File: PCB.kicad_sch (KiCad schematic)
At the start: 57 parts, among them J1 USB_C_Receptacle_USB2.0_16P, J10 Conn_01x05_Pin, J11 Conn_01x05_Pin, J12 Conn_01x03_Pin, J2 Conn_01x04_Pin, J3 Conn_01x04_Pin, J4 Conn_01x07_Pin, J5 Conn_01x02_Pin, J6 Conn_01x02_Pin, J7 Conn_01x02_Pin, J8 Conn_01x04_Pin, J9 Conn_01x07_Pin, SW1 SW_Push, SW2 SW_Push, U1 TMC2209_SILENTSTEPSTICK, U2 TMC2209_SILENTSTEPSTICK, U3 D3V3XA4B10LP, U4 AMS1117-3.3 (UMW), U5 TMC2209_SILENTSTEPSTICK, U6 ESP32-S3-WROOM-1

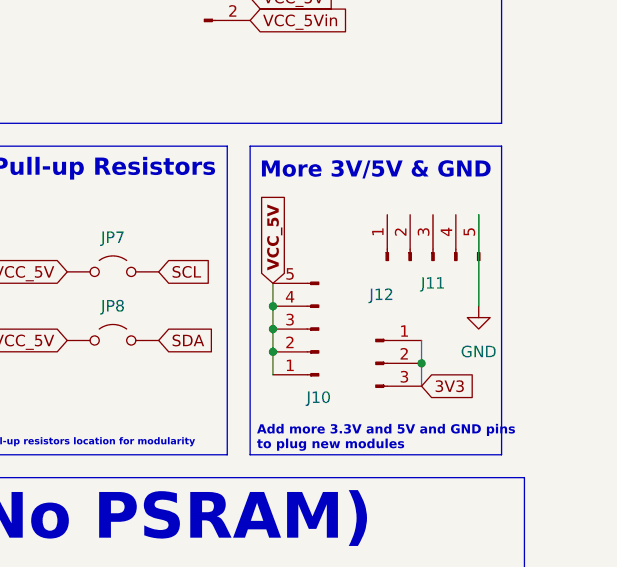
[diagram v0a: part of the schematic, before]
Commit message: Dernier DRC après modicifications
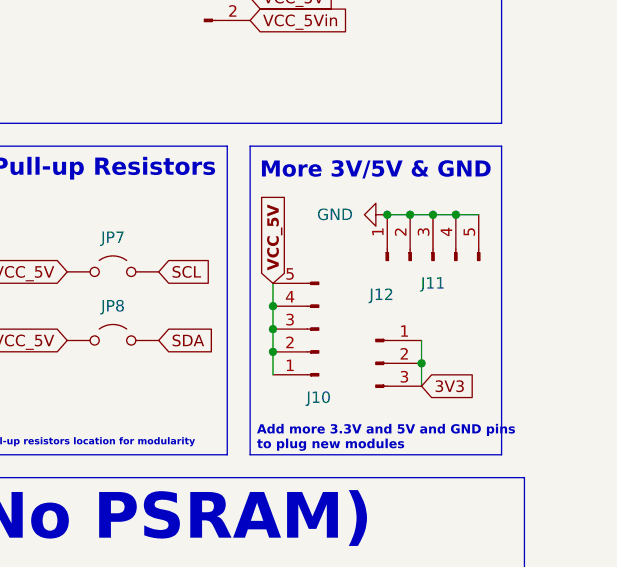
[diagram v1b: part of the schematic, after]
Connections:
- net GND: now also J11.1 (Pin_1), J11.2 (Pin_2), J11.3 (Pin_3), J11.4 (Pin_4)
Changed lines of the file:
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@@
 	)
 	(junction
+		(at 393.7 130.81)
+		(diameter 0)
+		(color 0 0 0 0)
+	)
+	(junction
 		(at 373.38 146.05)
 		(diameter 0)
@@
 	)
 	(junction
+		(at 386.08 130.81)
+		(diameter 0)
+		(color 0 0 0 0)
+	)
+	(junction
 		(at 290.83 176.53)
 		(diameter 0)
@@
 	)
 	(junction
+		(at 388.62 130.81)
+		(diameter 0)
+		(color 0 0 0 0)
+	)
+	(junction
 		(at 64.77 149.86)
 		(diameter 0)
@@
 	)
 	(junction
+		(at 391.16 130.81)
+		(diameter 0)
+		(color 0 0 0 0)
+	)
+	(junction
 		(at 373.38 143.51)
 		(diameter 0)
@@
 	(wire
 		(pts
+			(xy 388.62 130.81) (xy 391.16 130.81)
+		)
+		(stroke
+			(width 0)
+			(type default)
+		)
+	)
+	(wire
+		(pts
 			(xy 71.12 222.25) (xy 80.01 222.25)
 		)
@@
 	(wire
 		(pts
+			(xy 386.08 130.81) (xy 388.62 130.81)
+		)
+		(stroke
+			(width 0)
+			(type default)
+		)
+	)
+	(wire
+		(pts
 			(xy 71.12 222.25) (xy 71.12 223.52)
 		)
@@
 	(wire
 		(pts
+			(xy 393.7 130.81) (xy 396.24 130.81)
+		)
+		(stroke
+			(width 0)
+			(type default)
+		)
+	)
+	(wire
+		(pts
 			(xy 181.61 233.68) (xy 189.23 233.68)
 		)
@@
 	(wire
 		(pts
+			(xy 391.16 130.81) (xy 393.7 130.81)
+		)
+		(stroke
+			(width 0)
+			(type default)
+		)
+	)
+	(wire
+		(pts
 			(xy 74.93 58.42) (xy 80.01 58.42)
 		)
@@
 	(wire
 		(pts
-			(xy 396.24 130.81) (xy 396.24 140.97)
-		)
-		(stroke
-			(width 0)
-			(type default)
-		)
-	)
-	(wire
-		(pts
 			(xy 34.29 124.46) (xy 39.37 124.46)
 		)
@@
 	(symbol
 		(lib_id "power:GND")
-		(at 396.24 140.97 0)
+		(at 386.08 130.81 270)
 		(unit 1)
 		(exclude_from_sim no)
@@
 		(fields_autoplaced yes)
 		(property "Reference" "#PWR033"
-			(at 396.24 147.32 0)
+			(at 379.73 130.81 0)
 			(effects
 				(font
@@
 		)
 		(property "Value" "GND"
-			(at 396.24 146.05 0)
+			(at 382.27 130.8099 90)
 			(effects
 				(font
 					(size 1.27 1.27)
 				)
+				(justify right)
 			)
 		)
 		(property "Footprint" ""
-			(at 396.24 140.97 0)
+			(at 386.08 130.81 0)
 			(effects
 				(font
@@
 		)
 		(property "Datasheet" ""
-			(at 396.24 140.97 0)
+			(at 386.08 130.81 0)
 			(effects
 				(font
@@
 		)
 		(property "Description" "Power symbol creates a global label with name \"GND\" , ground"
-			(at 396.24 140.97 0)
+			(at 386.08 130.81 0)
 			(effects
 				(font

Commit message: Test DRC OK
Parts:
- C5: footprint Resistor_SMD:R_0603_1608Metric -> Capacitor_SMD:C_1206_3216Metric_Pad1.33x1.80mm_HandSolder
- R2, R3: footprint Resistor_SMD:R_01005_0402Metric -> Resistor_SMD:R_0805_2012Metric_Pad1.20x1.40mm_HandSolder
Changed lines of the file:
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@@
 			)
 		)
-		(property "Footprint" "Resistor_SMD:R_01005_0402Metric"
+		(property "Footprint" "Resistor_SMD:R_0805_2012Metric_Pad1.20x1.40mm_HandSolder"
 			(at 78.232 50.8 90)
 			(effects
@@
 			)
 		)
-		(property "Footprint" "Resistor_SMD:R_0603_1608Metric"
+		(property "Footprint" "Capacitor_SMD:C_1206_3216Metric_Pad1.33x1.80mm_HandSolder"
 			(at 122.8852 134.62 0)
 			(effects
@@
 			)
 		)
-		(property "Footprint" "Resistor_SMD:R_01005_0402Metric"
+		(property "Footprint" "Resistor_SMD:R_0805_2012Metric_Pad1.20x1.40mm_HandSolder"
 			(at 73.152 54.61 90)
 			(effects

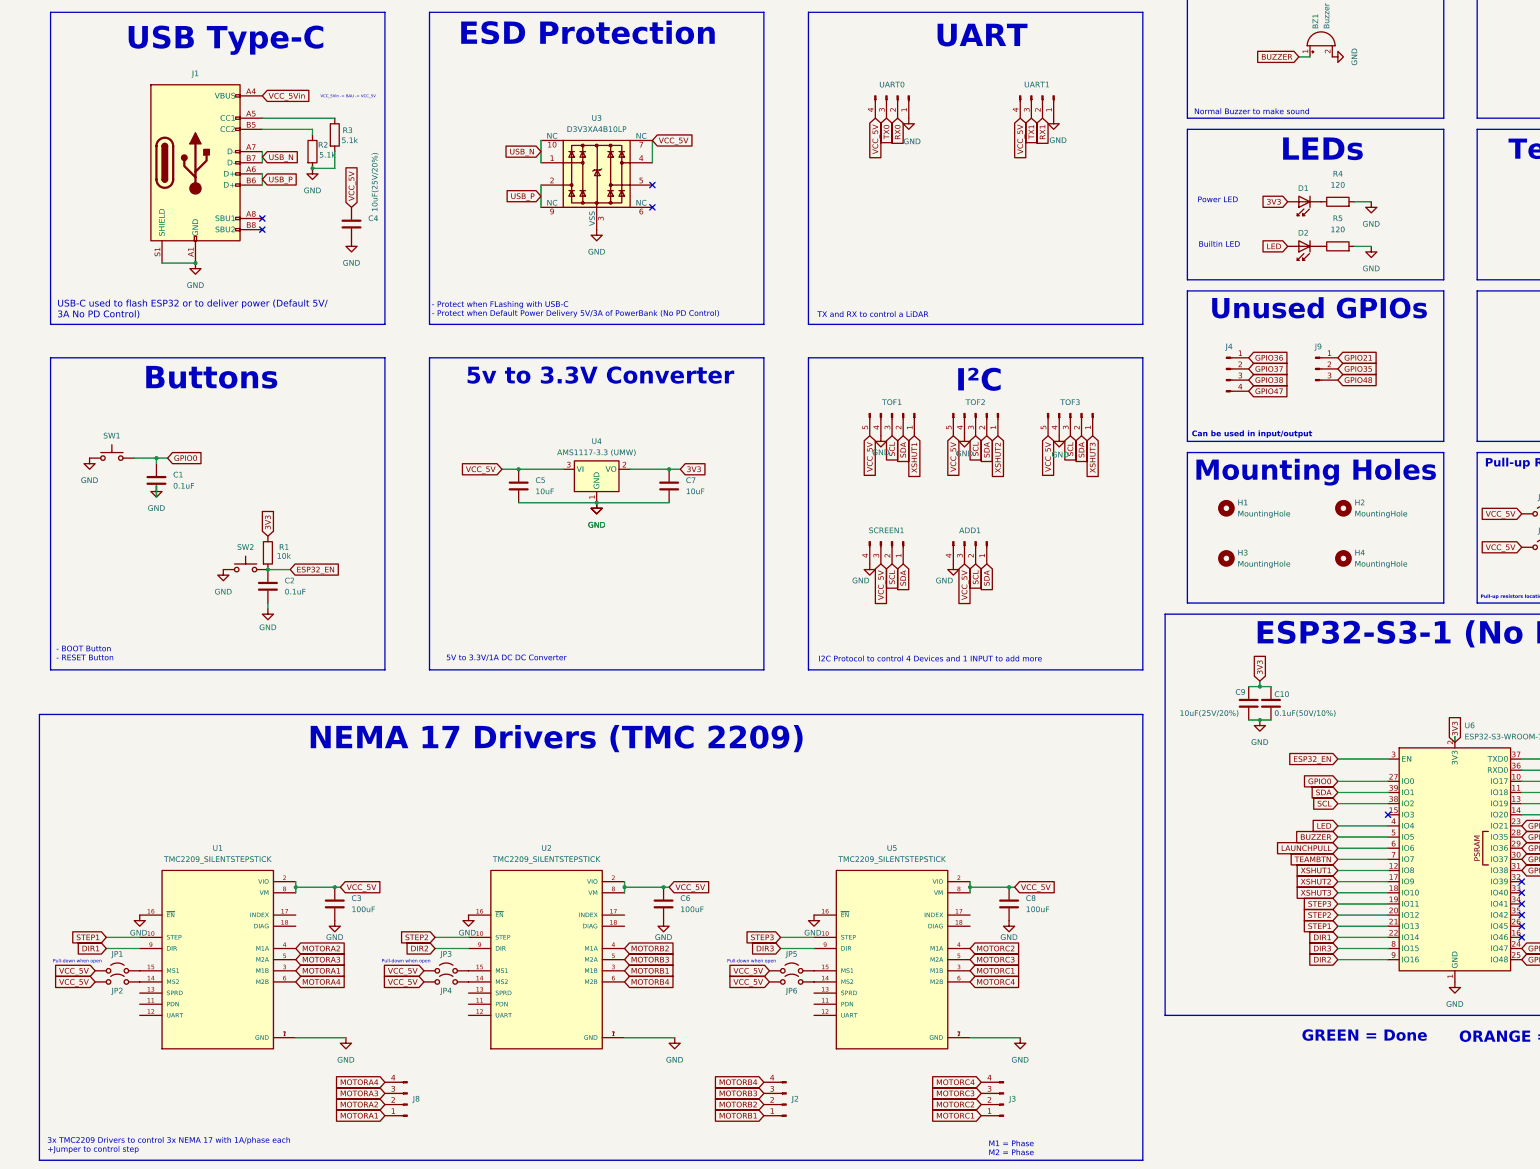
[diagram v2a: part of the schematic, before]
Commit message: V2 avec test DRC OK
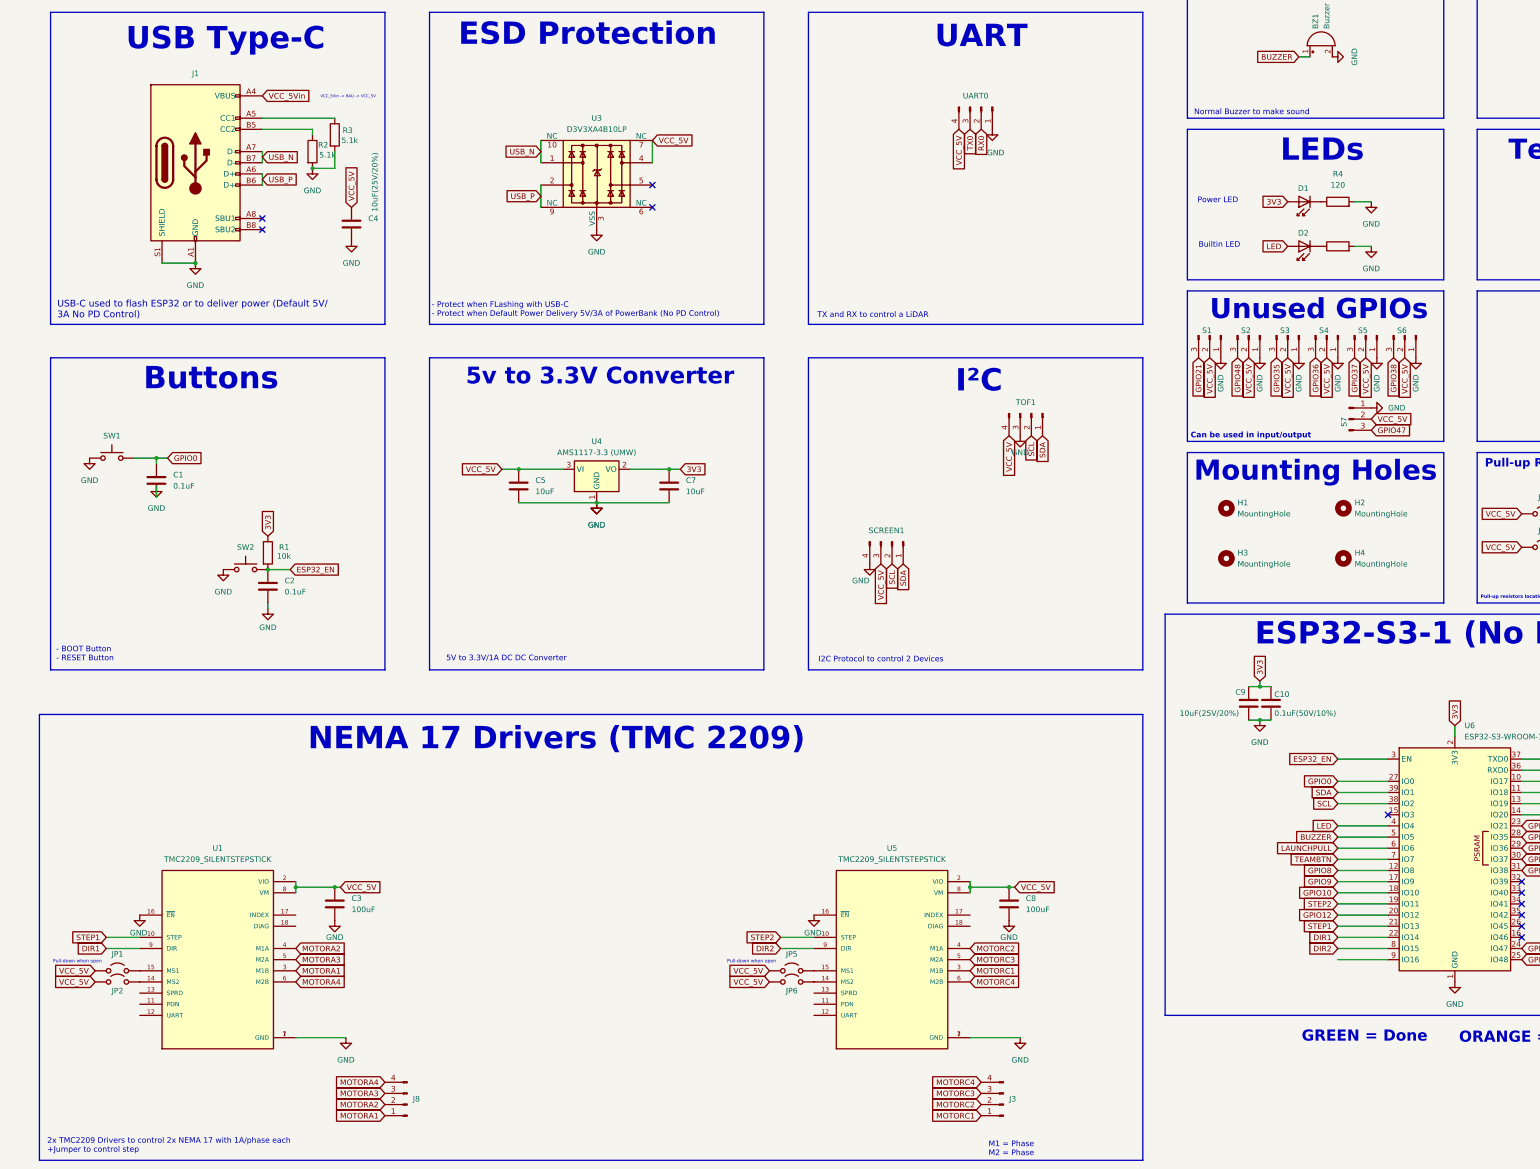
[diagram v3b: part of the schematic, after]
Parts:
- removed ADD1, J2, UART1: Conn_01x04_Pin, Connector_PinHeader_2.54mm:PinHeader_1x04_P2.54mm_Vertical, symbol Connector:Conn_01x04_Pin
- removed C6: 100uF, Capacitor_THT:CP_Radial_D10.0mm_P5.00mm, symbol Device:C
- removed J4: Conn_01x07_Pin, Connector_PinHeader_2.54mm:PinHeader_1x04_P2.54mm_Vertical, symbol Connector:Conn_01x04_Pin
- removed J9: Conn_01x07_Pin, Connector_PinHeader_2.54mm:PinHeader_1x03_P2.54mm_Vertical, symbol Connector:Conn_01x03_Pin
- removed JP3, JP4: Jumper_2_Open, Connector_PinHeader_2.54mm:PinHeader_1x02_P2.54mm_Vertical, symbol Jumper:Jumper_2_Open
- removed TOF1, TOF2, TOF3: Conn_01x05_Pin, Connector_PinHeader_2.54mm:PinHeader_1x05_P2.54mm_Vertical, symbol Connector:Conn_01x05_Pin
- removed U2: TMC2209_SILENTSTEPSTICK, TMC2209:MODULE_TMC2209_SILENTSTEPSTICK, symbol TMC2209_SILENTSTEPSTICK:TMC2209_SILENTSTEPSTICK
- added S1, S2, S3, S4, S5, S6, S7: Conn_01x07_Pin, Connector_PinHeader_2.54mm:PinHeader_1x03_P2.54mm_Vertical, symbol Connector:Conn_01x03_Pin
- added TOF1: Conn_01x04_Pin, Connector_PinHeader_2.54mm:PinHeader_1x04_P2.54mm_Vertical, symbol Connector:Conn_01x04_Pin
- C1, C10, C2, C4, C9, R4, R5: footprint Resistor_SMD:R_01005_0402Metric -> Resistor_SMD:R_0805_2012Metric_Pad1.20x1.40mm_HandSolder
- C7: footprint Resistor_SMD:R_0603_1608Metric -> Capacitor_SMD:C_1206_3216Metric_Pad1.33x1.80mm_HandSolder
- D1, D2: footprint LED_SMD:LED_0603_1608Metric -> LED_SMD:LED_0805_2012Metric_Pad1.15x1.40mm_HandSolder
- R1: footprint Resistor_SMD:R_01005_0402Metric -> Resistor_SMD:R_1206_3216Metric_Pad1.30x1.75mm_HandSolder
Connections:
- net DIR3 is gone; now on net DIR2: U5.9 (DIR), U6.8 (IO15)
- net STEP3 is gone; now on net STEP2: U5.10 (STEP), U6.19 (IO11)
- net DIR2: no longer U6.9 (IO16)
- net GND: now also S1.1 (Pin_1), S2.1 (Pin_1), S3.1 (Pin_1), S4.1 (Pin_1), S5.1 (Pin_1), S6.1 (Pin_1), S7.1 (Pin_1), TOF1.3 (Pin_3)
- net GPIO21: now also S1.3 (Pin_3)
- net GPIO35: now also S3.3 (Pin_3)
- net GPIO36: now also S4.3 (Pin_3)
- net GPIO37: now also S5.3 (Pin_3)
- net GPIO38: now also S6.3 (Pin_3)
- net GPIO47: now also S7.3 (Pin_3)
- net GPIO48: now also S2.3 (Pin_3)
- net SCL: now also TOF1.2 (Pin_2)
- net SDA: now also TOF1.1 (Pin_1)
- net STEP2: no longer U6.20 (IO12)
- net VCC_5V: now also S1.2 (Pin_2), S2.2 (Pin_2), S3.2 (Pin_2), S4.2 (Pin_2), S5.2 (Pin_2), S6.2 (Pin_2), S7.2 (Pin_2), TOF1.4 (Pin_4)
- net XSHUT1 renamed GPIO8
- net XSHUT2 renamed GPIO9
- net XSHUT3 renamed GPIO10
- new net GPIO12: U6.20 (IO12)
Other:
- note added: "2x TMC2209 Drivers to control 2x NEMA 17 with 1A/phase each +Jumper to control step"
- note added: "I2C Protocol to control 2 Devices"
- note removed: "3x TMC2209 Drivers to control 3x NEMA 17 with 1A/phase each +Jumper to control step"
- note removed: "I2C Protocol to control 4 Devices and 1 INPUT to add more"
- moved on the sheet: UART0

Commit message: debut V3
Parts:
- removed BZ1: Buzzer, Buzzer_Beeper:Buzzer_12x9.5RM7.6, symbol Device:Buzzer
- removed D2: ~, LED_SMD:LED_0805_2012Metric_Pad1.15x1.40mm_HandSolder, symbol LED:SFH482
- removed H1, H2, H3, H4: MountingHole, MountingHole:MountingHole_3.2mm_M3, symbol Mechanical:MountingHole
- removed J10, J11: Conn_01x05_Pin, Connector_PinHeader_2.54mm:PinHeader_1x05_P2.54mm_Vertical, symbol Connector:Conn_01x05_Pin
- removed J12: Conn_01x03_Pin, Connector_PinHeader_2.54mm:PinHeader_1x03_P2.54mm_Vertical, symbol Connector:Conn_01x03_Pin
- removed JP5, JP6: Jumper_2_Open, Connector_PinHeader_2.54mm:PinHeader_1x02_P2.54mm_Vertical, symbol Jumper:Jumper_2_Open
- removed JP7, JP8: Jumper_2_Open, Resistor_SMD:R_1206_3216Metric_Pad1.30x1.75mm_HandSolder, symbol Jumper:Jumper_2_Open
- removed S1, S2, S3, S4, S5, S6, S7: Conn_01x07_Pin, Connector_PinHeader_2.54mm:PinHeader_1x03_P2.54mm_Vertical, symbol Connector:Conn_01x03_Pin
- removed SCREEN1, TOF1: Conn_01x04_Pin, Connector_PinHeader_2.54mm:PinHeader_1x04_P2.54mm_Vertical, symbol Connector:Conn_01x04_Pin
- removed U3: D3V3XA4B10LP, Package_DFN_QFN:Diodes_UDFN-10_1.0x2.5mm_P0.5mm, symbol Power_Protection:D3V3XA4B10LP
- added D2: SMLVN6RGB, LED_SMD:LED_RGB_5050-6, symbol LED:SMLVN6RGB
- added F1: Fuse, Fuse:Fuse_1206_3216Metric, symbol Device:Fuse
- added H1, H2, H3, H4: MountingHole_Pad, MountingHole:MountingHole_3.2mm_M3_Pad, symbol Mechanical:MountingHole_Pad
- added J13, J4, J9: Conn_01x06_Pin, Connector_PinHeader_2.54mm:PinHeader_1x06_P2.54mm_Vertical, symbol Connector:Conn_01x06_Pin
- added JP3, JP4: Jumper_2_Open, Connector_PinHeader_2.54mm:PinHeader_1x02_P2.54mm_Vertical, symbol Jumper:Jumper_2_Open
- added R6: 10k, Resistor_SMD:R_1206_3216Metric_Pad1.30x1.75mm_HandSolder, symbol Device:R
- added R7, R8, R9: 120, Resistor_SMD:R_0805_2012Metric_Pad1.20x1.40mm_HandSolder, symbol Device:R
- added SCREEN2, TOF2, UART1: Conn_01x04_Pin, Connector_PinHeader_2.54mm:PinHeader_1x04_P2.54mm_Vertical, symbol Connector:Conn_01x04_Pin
- added U2: USBLC6-2SC6, Package_TO_SOT_SMD:SOT-23-6_Handsoldering, symbol Power_Protection:USBLC6-2SC6
- R5: value 120 -> 10k; footprint Resistor_SMD:R_0805_2012Metric_Pad1.20x1.40mm_HandSolder -> Resistor_SMD:R_1206_3216Metric_Pad1.30x1.75mm_HandSolder
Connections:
- net GPIO35 is gone; now on net STEP1: U6.28 (IO35)
- net GPIO36 is gone; now on net DIR1: U6.29 (IO36)
- net GPIO37 is gone; now on net STEP2: U6.30 (IO37)
- net GPIO38 is gone; now on net DIR2: U6.31 (IO38)
- net DIR1: no longer U6.22 (IO14)
- net DIR2: no longer U6.8 (IO15)
- net GND: now also D2.4 (GK), D2.5 (RK), D2.6 (BK), H1.1, H2.1, H3.1, H4.1, J13.1 (Pin_1), J13.2 (Pin_2), J13.3 (Pin_3), J13.4 (Pin_4), J13.5 (Pin_5), J13.6 (Pin_6), SCREEN2.4 (Pin_4), TOF2.3 (Pin_3), U2.2 (GND), UART1.1 (Pin_1); no longer R5.2
- net GPIO21: now also J4.6 (Pin_6)
- net GPIO9: now also J4.4 (Pin_4)
- net RX1: now also UART1.2 (Pin_2)
- net SCL: now also R5.2, SCREEN2.2 (Pin_2), TOF2.2 (Pin_2)
- net SDA: now also R6.2, SCREEN2.1 (Pin_1), TOF2.1 (Pin_1)
- net STEP1: no longer U6.21 (IO13)
- net STEP2: no longer U6.19 (IO11)
- net TX1: now also UART1.3 (Pin_3)
- net USB_N: now also U2.4 (I/O2); no longer J1.A7 (D-), J1.B7 (D-)
- net USB_P: now also U2.6 (I/O1); no longer J1.A6 (D+), J1.B6 (D+)
- net VCC_5V: now also R5.1, J9.1 (Pin_1), J9.2 (Pin_2), J9.3 (Pin_3), J9.4 (Pin_4), J9.5 (Pin_5), J9.6 (Pin_6), JP3.1 (A), JP4.1 (A), R6.1, SCREEN2.3 (Pin_3), TOF2.4 (Pin_4), U2.5 (VBUS), UART1.4 (Pin_4)
- net VCC_5Vin: now also F1.1; no longer J6.2 (Pin_2)
- net at U5.15 (MS1): now also JP3.2 (B)
- net GPIO16_PWM: now reaches U6.9 (IO16)
- net GPIO16_PWM: now also J4.1 (Pin_1)
- net at U5.14 (MS2): now also JP4.2 (B)
- net BUZZER renamed GPIO5
- net GPIO5: now also J4.5 (Pin_5)
- net GPIO0 renamed BOOT
- net GPIO12 renamed GPIO12_PWM
- net GPIO12_PWM: now also R8.1
- net LED renamed GPIO4
- new net: D2.3 (GA), R9.2
- new net: D2.1 (BA), R7.2
- new net: D2.2 (RA), R8.2
- new net GPIO11_PWM: R7.1, U6.19 (IO11)
- new net GPIO13_PWM: R9.1, U6.21 (IO13)
- new net GPIO14_PWM: J4.3 (Pin_3), U6.22 (IO14)
- new net GPIO15_PWM: J4.2 (Pin_2), U6.8 (IO15)
- new net USB_N_in: J1.A7 (D-), J1.B7 (D-), U2.3 (I/O2)
- new net USB_P_in: J1.A6 (D+), J1.B6 (D+), U2.1 (I/O1)
- new net VCC_5Vout: F1.2, J6.2 (Pin_2)
- no-connect marks 11 -> 9
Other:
- note added: "Analog(PWM)"
- note added: "F0 : I/O/T PINS"
- note added: "F1 : I/O/T PINS"
- note added: "Fuse"
- note added: "GPIO 43"
- note added: "GPIO 44"
- note added: "Pull-up Resistors I2C"
- note added: "Unused GPIOs F0 (I/O/T)"
- note added: "Unused GPIOs F1 (I/O/T)"
- note added: "VCC_5Vin -> Fuse -> VCC_5out -> BAU -> VCC_5V"
- note added: "}"
- note removed: "Add more 3.3V and 5V and GND pins to plug new modules"
- note removed: "Builtin LED"
- note removed: "Buzzer"
- note removed: "Can be used in input/output"
- note removed: "M1 = Phase M2 = Phase"
- note removed: "More 3V/5V & GND"
- note removed: "Normal Buzzer to make sound"
- note removed: "Pull-up Resistors"
- note removed: "Unused GPIOs"
- note removed: "VCC_5Vin -> BAU -> VCC_5V"
- moved on the sheet: C1, C10, C2, C3, C5, C7, C8, C9, D1, J1, J3, J5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
